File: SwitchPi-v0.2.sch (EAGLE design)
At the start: 10 parts, among them IC1 MCP23017SP, IC2 MCP2300X/P, P2 P2, P3 P3

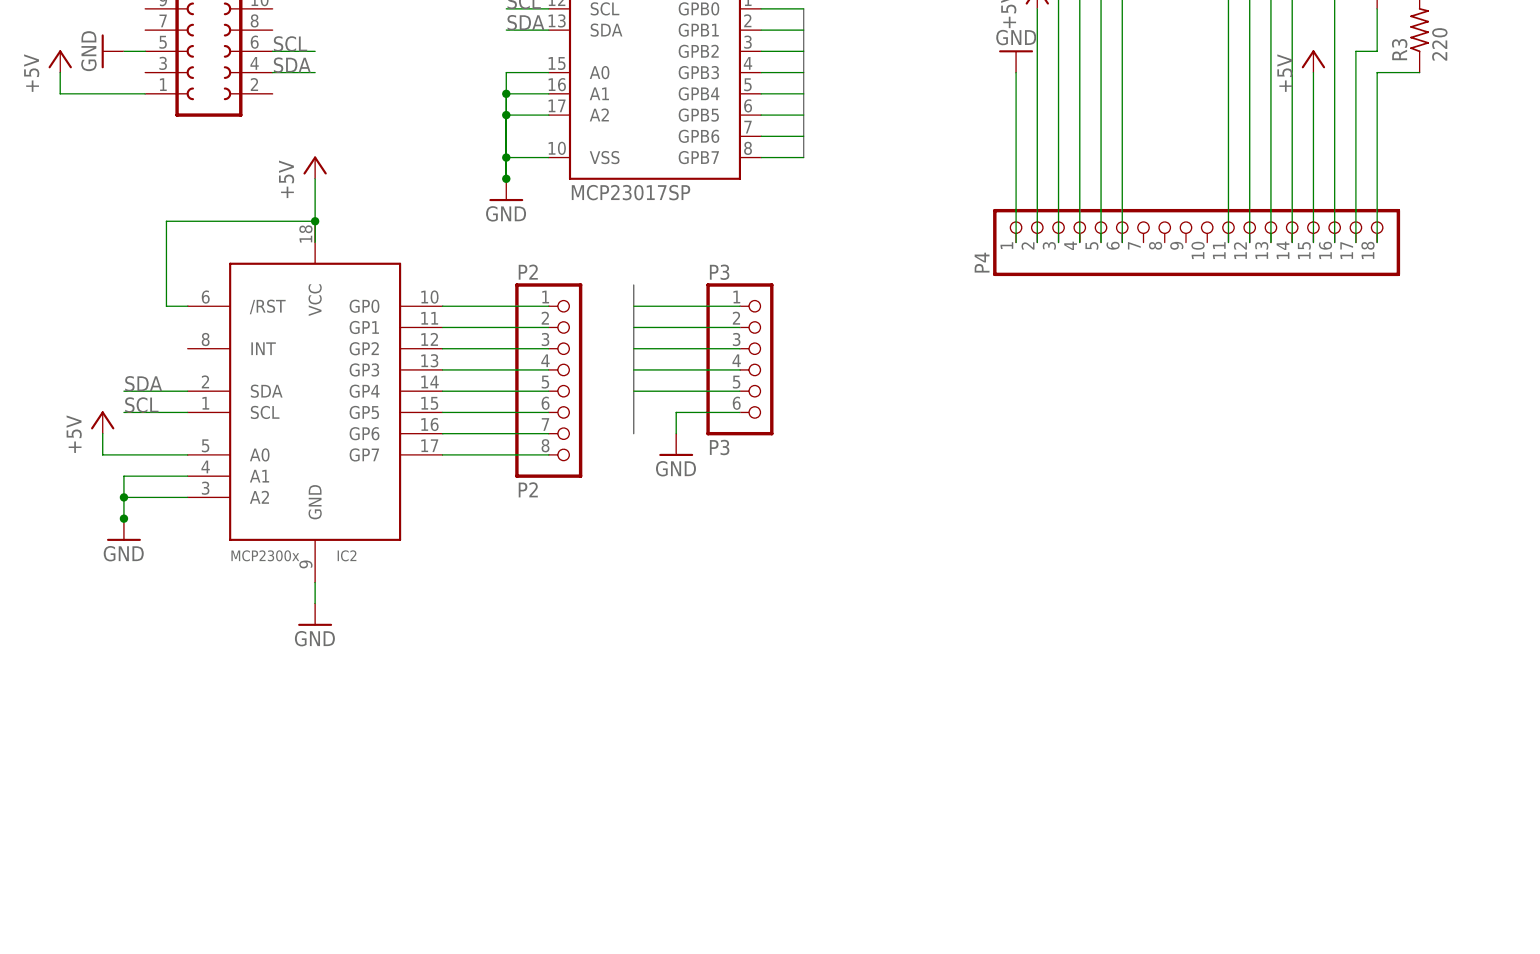
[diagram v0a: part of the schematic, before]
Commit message: updates
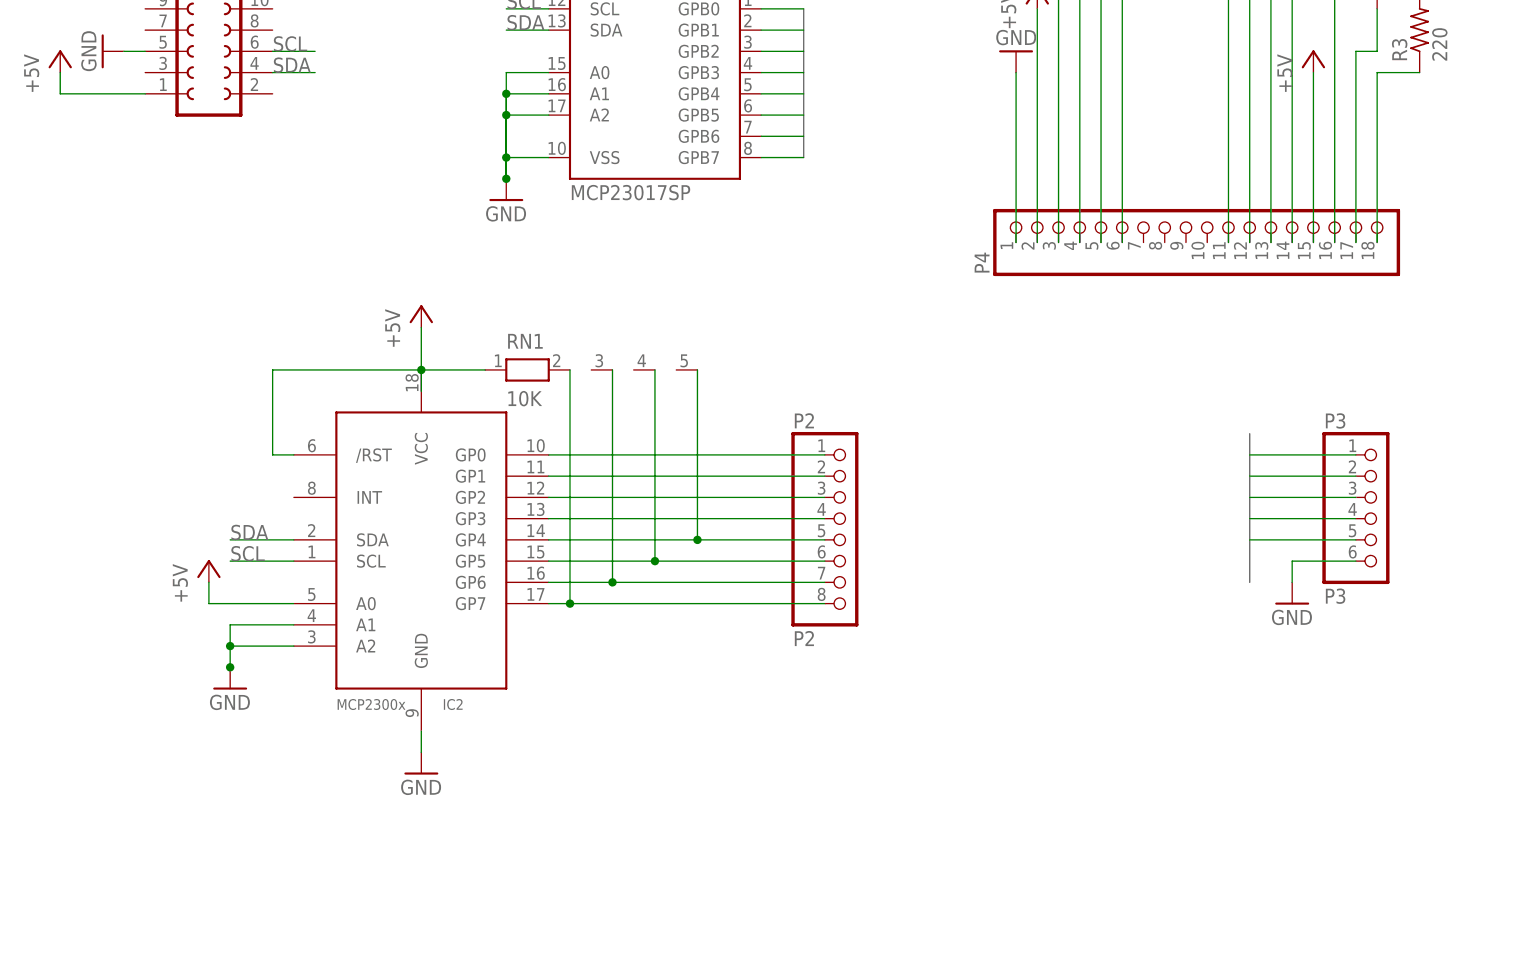
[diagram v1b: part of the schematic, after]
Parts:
- added RN1: 10K, resistor-net:RN04
- P4: device adafruit:PINHD-1X18 -> adafruit:PINHD-1X18-BIG
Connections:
- net +5V: now also RN1.1
- net N$10: now also RN1.2
- net N$7: now also RN1.5
- net N$8: now also RN1.4
- net N$9: now also RN1.3
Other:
- moved on the sheet: IC2, P2, P3
